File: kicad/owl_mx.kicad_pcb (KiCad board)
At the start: 2 copper layers, 152.1 x 123.2 mm, 46 parts

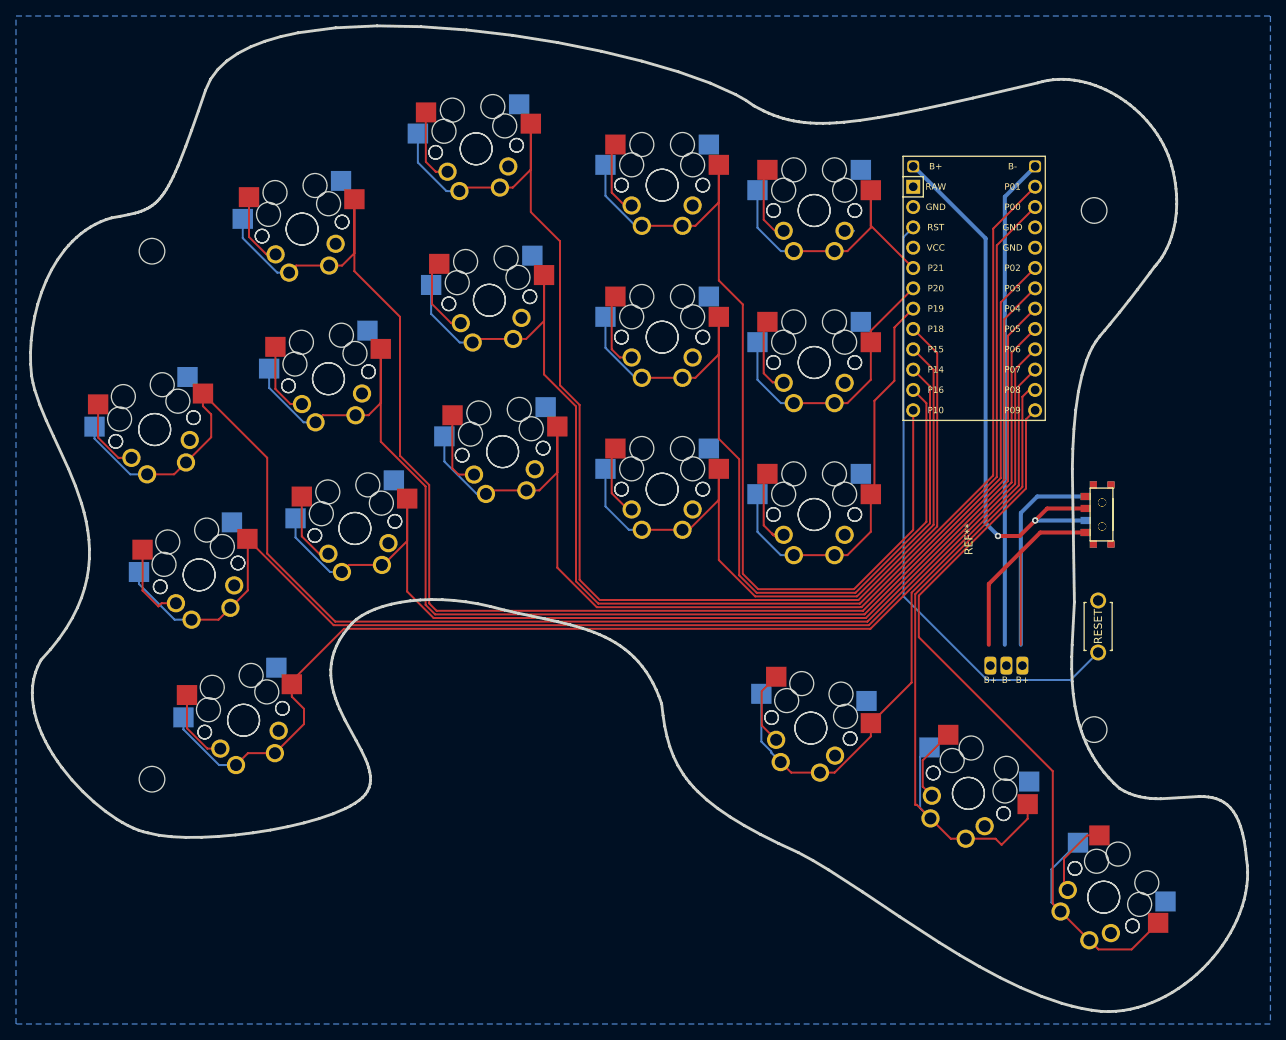
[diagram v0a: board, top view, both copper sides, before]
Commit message: in progress
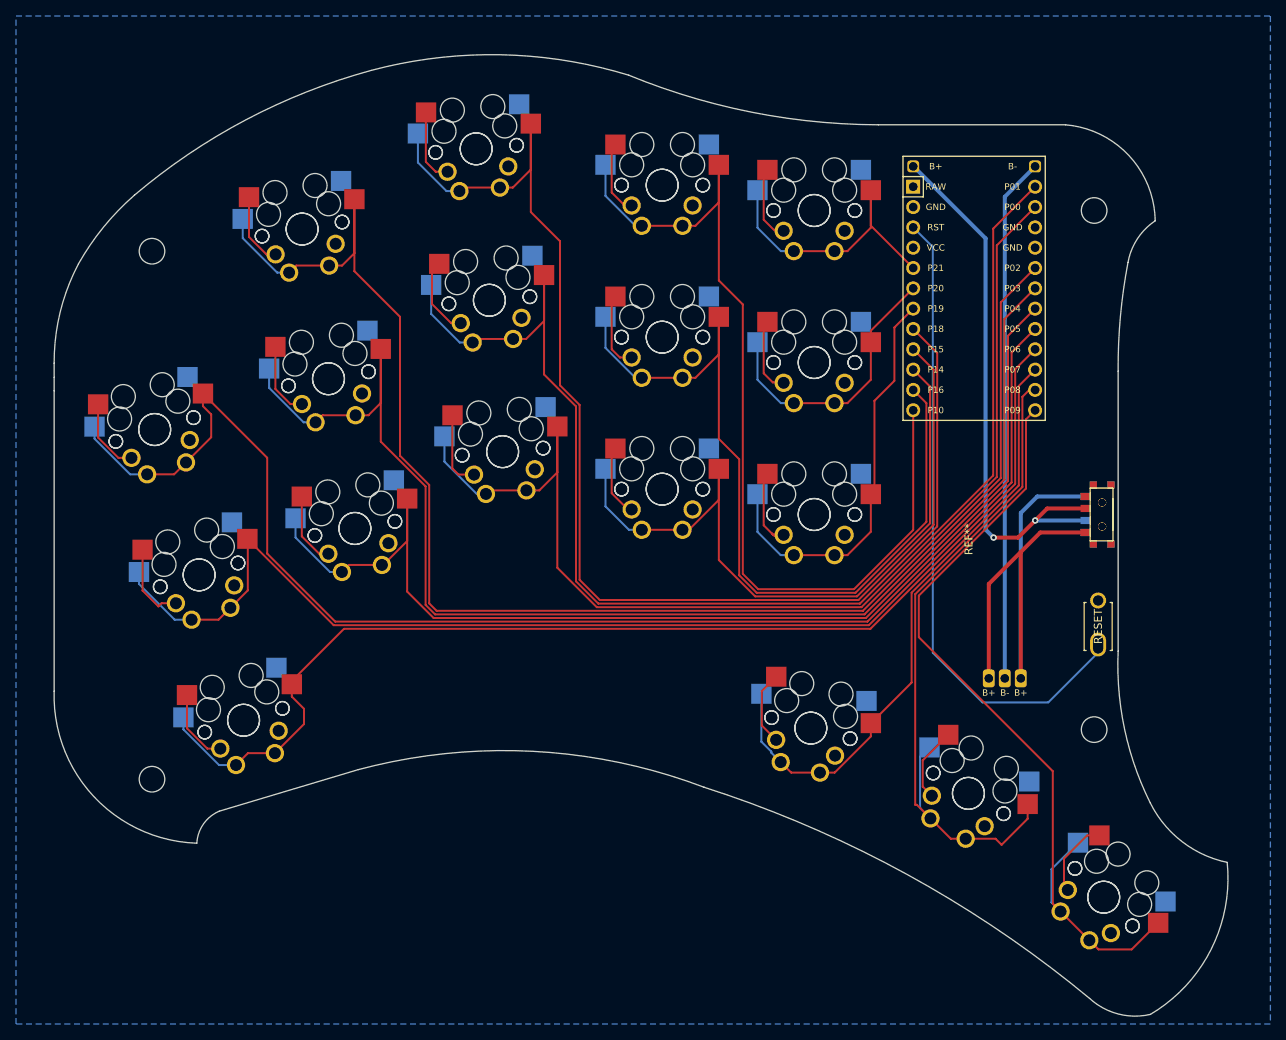
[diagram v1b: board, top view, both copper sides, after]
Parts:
- moved ? 1.61 mm to (157.6, -54.4)
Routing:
- net Braw: track 59.4 -> 72.0 mm
- net Bminus: track 61.4 -> 65.6 mm
- net RST: track 76.7 -> 80.0 mm
- net GND: track 172.9 -> 170.5 mm
- net Bplus: track 69.3 -> 69.9 mm
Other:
- board size 152.1 x 123.2 mm -> 146.7 x 120.2 mm
